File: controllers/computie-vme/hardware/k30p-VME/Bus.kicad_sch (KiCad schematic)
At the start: 30 parts, among them U17 VME64-P1-3R

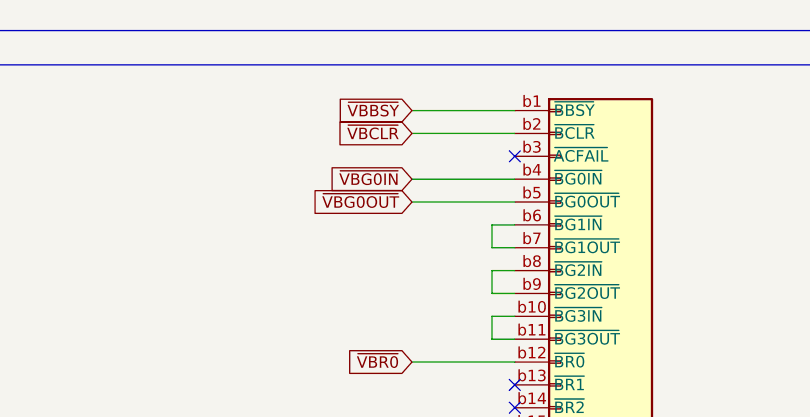
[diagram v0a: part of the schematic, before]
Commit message: k30p-VME rev.1, MemBird Woodcock rev.1, and frontpanels
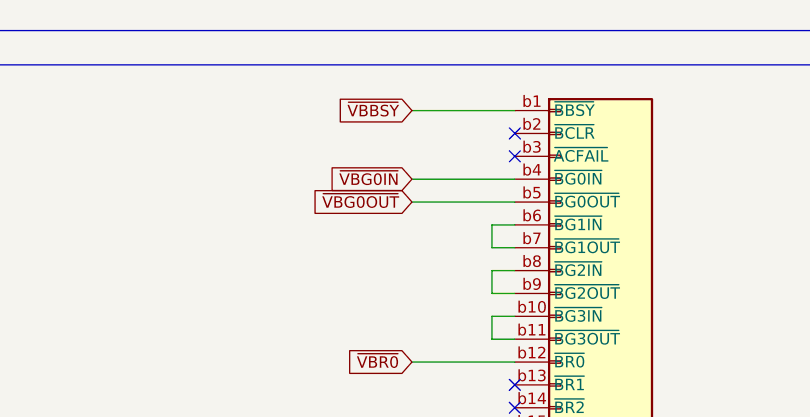
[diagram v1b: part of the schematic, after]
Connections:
- net ~{VBCLR}: no longer names the net of U17.b2 (~{BCLR})
- no-connect marks 12 -> 13
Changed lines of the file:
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@@
 	)
 	(no_connect
+		(at 153.67 26.67)
+	)
+	(no_connect
 		(at 153.67 77.47)
 	)
@@
 	(wire
 		(pts
-			(xy 142.24 26.67) (xy 153.67 26.67)
-		)
-		(stroke
-			(width 0)
-			(type default)
-		)
-	)
-	(wire
-		(pts
 			(xy 214.63 118.11) (xy 224.79 118.11)
 		)
@@
 				)
 				(justify right)
-				(hide yes)
 			)
 		)
@@
 				)
 				(justify right)
-				(hide yes)
 			)
 		)
@@
 				)
 				(justify right)
-				(hide yes)
 			)
 		)
@@
 				)
 				(justify right)
-				(hide yes)
 			)
 		)
@@
 				)
 				(justify left)
-				(hide yes)
 			)
 		)
@@
 				)
 				(justify right)
-				(hide yes)
 			)
 		)
@@
 				)
 				(justify right)
-				(hide yes)
 			)
 		)
@@
 				)
 				(justify left)
-				(hide yes)
 			)
 		)
@@
 				)
 				(justify right)
-				(hide yes)
 			)
 		)
@@
 				)
 				(justify right)
-				(hide yes)
 			)
 		)
@@
 				)
 				(justify right)
-				(hide yes)
 			)
 		)
@@
 				)
 				(justify left)
-				(hide yes)
-			)
-		)
-	)
-	(global_label "~{VBCLR}"
-		(shape input)
-		(at 142.24 26.67 180)
-		(fields_autoplaced yes)
-		(effects
-			(font
-				(size 1.27 1.27)
-			)
-			(justify right)
-		)
-		(property "Intersheetrefs" "${INTERSHEET_REFS}"
-			(at 133.3281 26.67 0)
-			(effects
-				(font
-					(size 1.27 1.27)
-				)
-				(justify right)
-				(hide yes)
 			)
 		)
@@
 				)
 				(justify right)
-				(hide yes)
 			)
 		)
@@
 				)
 				(justify right)
-				(hide yes)
 			)
 		)
@@
 				)
 				(justify right)
-				(hide yes)
 			)
 		)
@@
 				)
 				(justify right)
-				(hide yes)
 			)
 		)
@@
 				)
 				(justify right)
-				(hide yes)
 			)
 		)
@@
 				)
 				(justify right)
-				(hide yes)
 			)
 		)
@@
 				)
 				(justify right)
-				(hide yes)
 			)
 		)
@@
 				)
 				(justify right)
-				(hide yes)
 			)
 		)
@@
 				)
 				(justify right)
-				(hide yes)
 			)
 		)
@@
 				)
 				(justify right)
-				(hide yes)
 			)
 		)
@@
 				)
 				(justify right)
-				(hide yes)
 			)
 		)
@@
 				)
 				(justify right)
-				(hide yes)
 			)
 		)
@@
 				)
 				(justify right)
-				(hide yes)
 			)
 		)
@@
 				)
 				(justify right)
-				(hide yes)
 			)
 		)
@@
 				)
 				(justify right)
-				(hide yes)
 			)
 		)
@@
 				)
 				(justify right)
-				(hide yes)
 			)
 		)
@@
 				)
 				(justify right)
-				(hide yes)
 			)
 		)
@@
 				)
 				(justify right)
-				(hide yes)
 			)
 		)
@@
 				)
 				(justify right)
-				(hide yes)
 			)
 		)
